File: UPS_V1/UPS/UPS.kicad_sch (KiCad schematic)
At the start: 83 parts, among them J1 Conn_01x02_Pin, J2 Conn_01x02_Pin, J3 USB_B_Micro, J4 Conn_01x02_Socket, J5 Conn_01x02_Pin, J6 Conn_01x02_Socket, J7 Conn_01x02_Pin, J8 PROVISIONAL_PORTS, U1 MT3608, U2 BQ24040DSQR, U3 LM2903, U4 TPS22810DRV, U5 LM285D-1.2

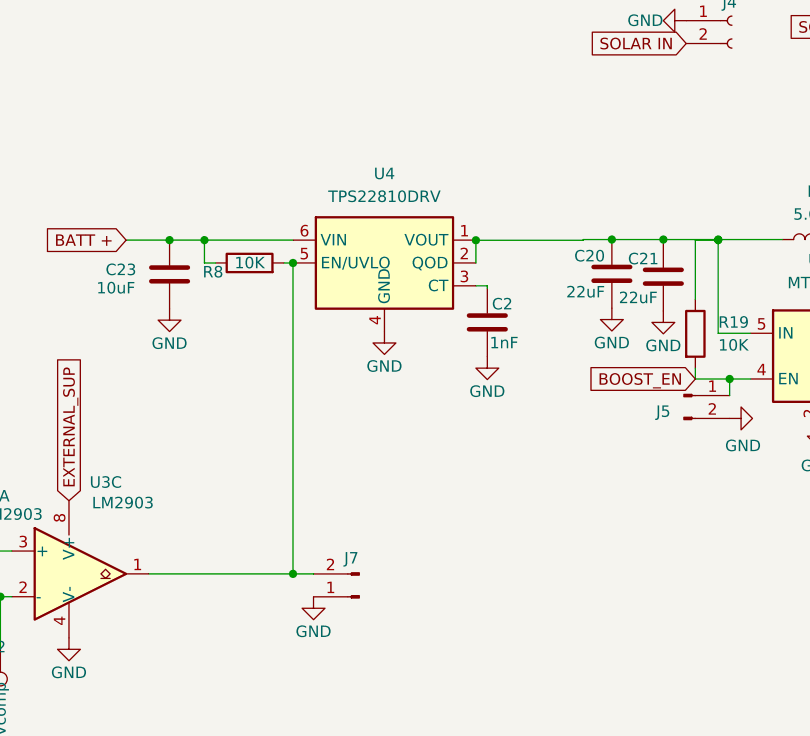
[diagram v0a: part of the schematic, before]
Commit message: -
updated symbol and footprint
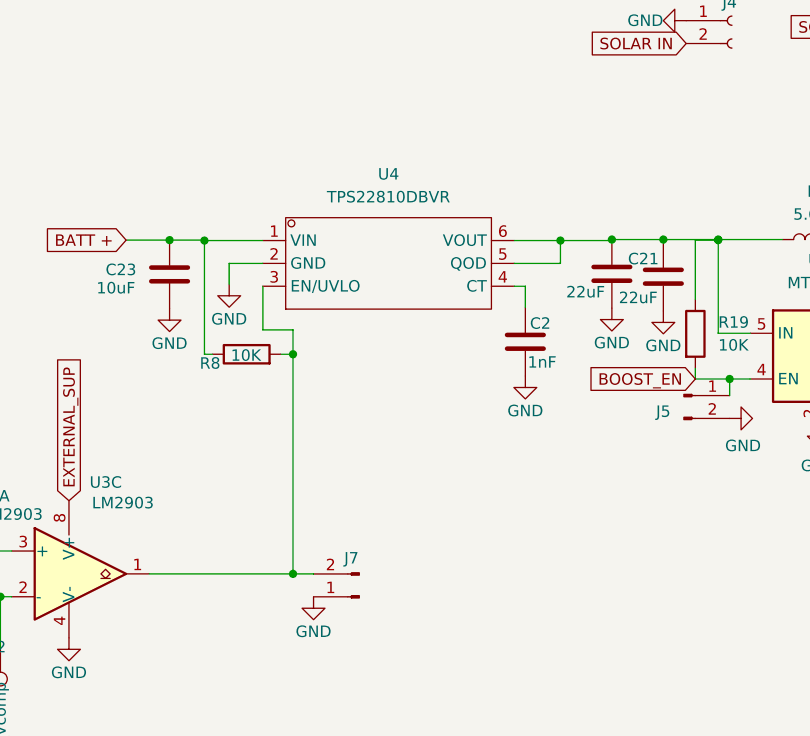
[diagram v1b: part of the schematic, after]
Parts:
- C15, C8: footprint Capacitor_SMD:C_0201_0603Metric_Pad0.64x0.40mm_HandSolder -> Capacitor_SMD:C_0603_1608Metric_Pad1.08x0.95mm_HandSolder
- U4: value TPS22810DRV -> TPS22810DBVR; footprint Package_SON:WSON-6-1EP_2x2mm_P0.65mm_EP1x1.6mm -> InnovationCentral:SOT-23-6_L2.9-W1.6-P0.95-LS2.8-BL; symbol Power_Management:TPS22810DRV -> 2024-09-10_13-19-56:TPS22810DBVR
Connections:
- net BATT +: now also U4.1 (VIN); no longer U4.6 (VIN)
- net GND: now also U4.2 (GND); no longer U4.4 (GND), U4.7 (GND)
- net at C20.1, C21.1, L4.1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: now also U4.5 (QOD), U4.6 (VOUT); no longer U4.1 (VOUT), U4.2 (QOD)
- net at U4.3 (EN/UVLO): now also J7.2 (Pin_2), R8.2, U3.1; no longer C2.2
- new net: C2.2, U4.4 (CT)
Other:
- moved on the sheet: C2, R8, U4
